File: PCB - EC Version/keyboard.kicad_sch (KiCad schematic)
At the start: 98 parts, among them J1 HRO_TYPE-C-31-M-12, J2 Conn_01x03, SW1 Alps SKRK, SW2 Alps SKRK, U1 TLV75533PDBV, U101 RP2040, U103 W25Q16, Y1 12MHz 3225 20pF

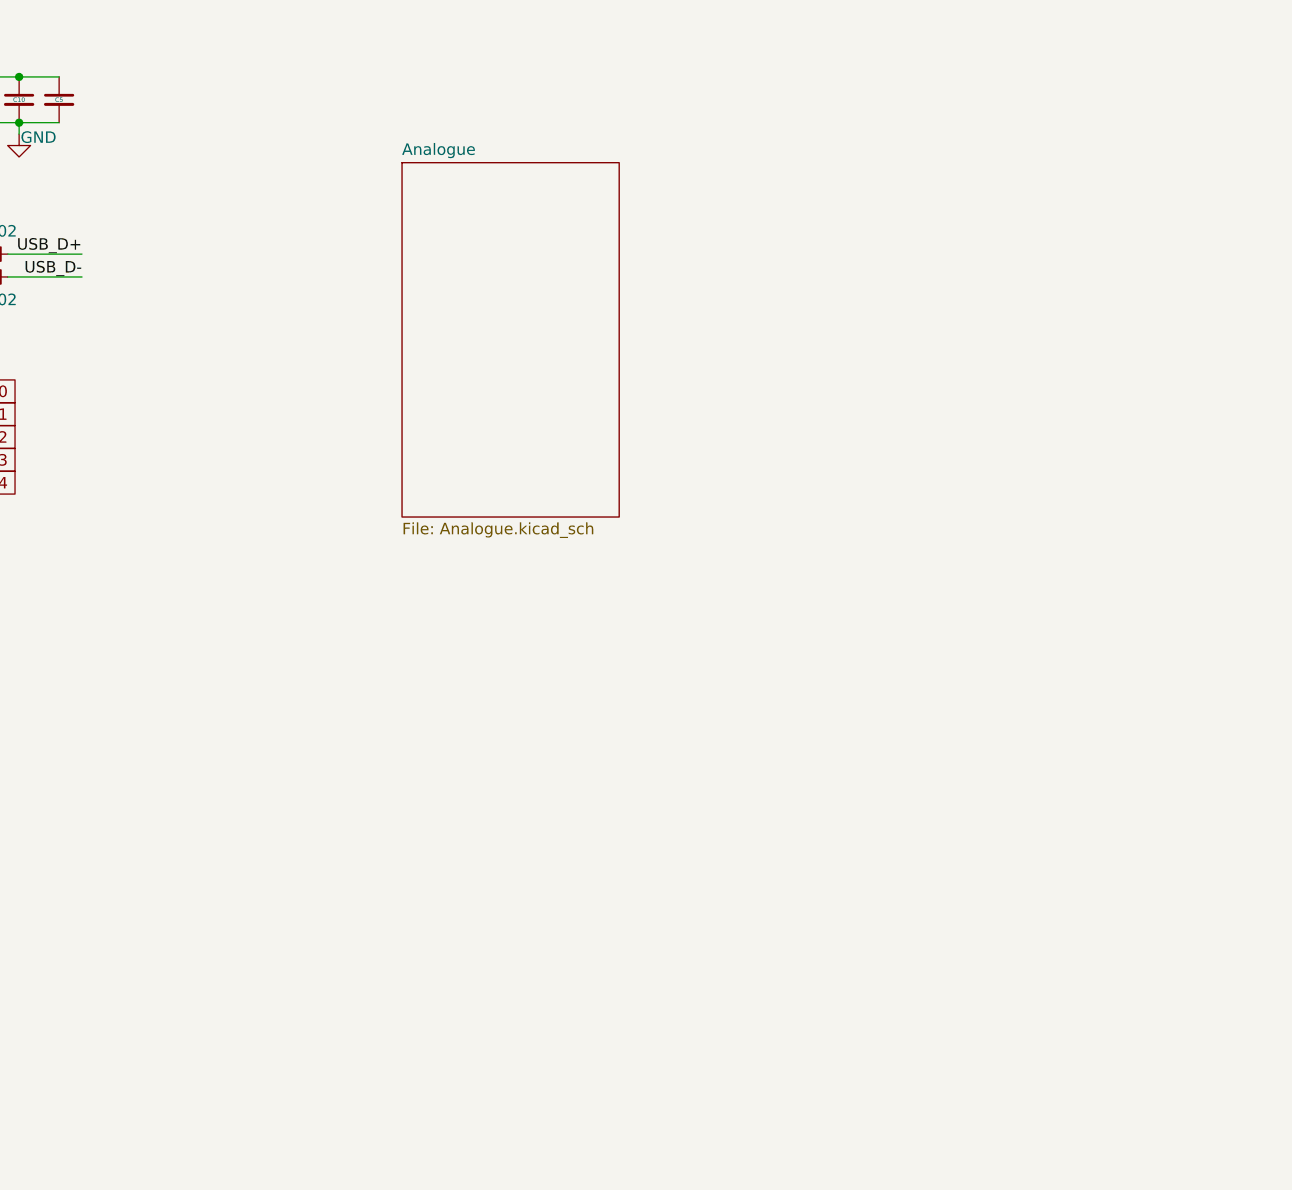
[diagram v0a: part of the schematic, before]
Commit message: couple extra bits
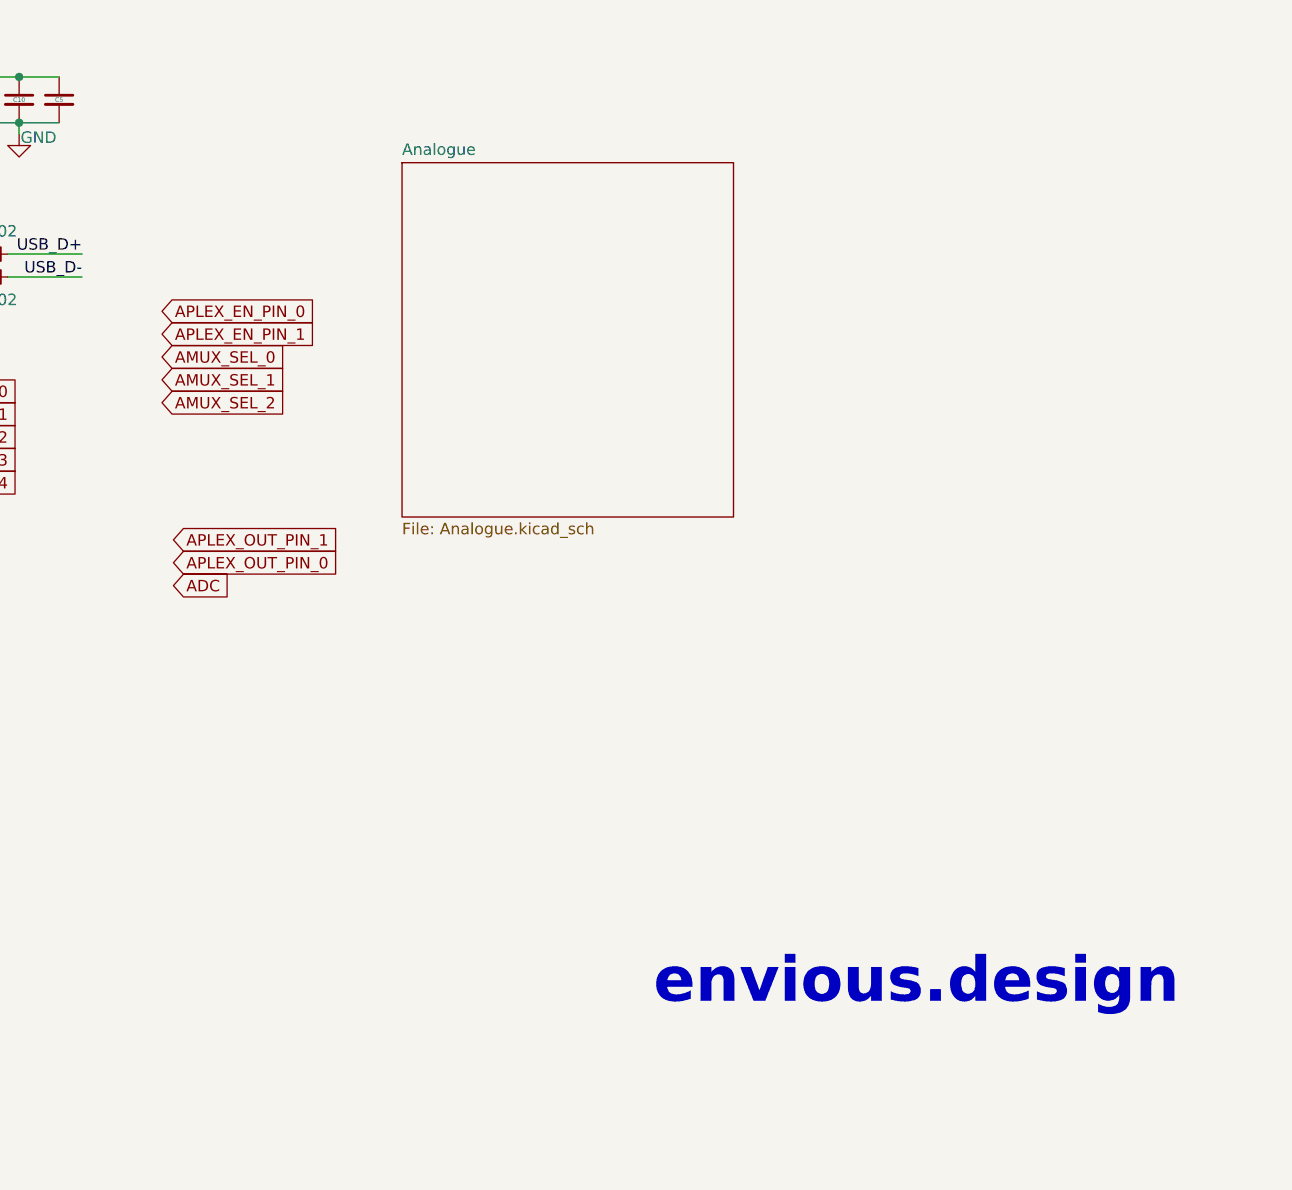
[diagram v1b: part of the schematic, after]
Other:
- note added: "envious.design"
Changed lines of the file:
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@@
     )
   )
+  (text "envious.design" (at 359.41 262.89 0)
+    (effects (font (face "Dissolve light") (size 5 5) (thickness 1) bold) (justify left bottom) (href "http://envious.design"))
+  )
   (label "USB_D+" (at 53.975 200.66 180) (fields_autoplaced)
     (effects (font (size 1.27 1.27)) (justify right bottom))
@@
     (effects (font (size 1.27 1.27)) (justify right bottom))
   )
+  (global_label "ADC" (shape input) (at 306.07 215.9 0) (fields_autoplaced)
+    (effects (font (size 1.27 1.27)) (justify left))
+    (property "Intersheetrefs" "${INTERSHEET_REFS}" (at 312.1117 215.8206 0)
+      (effects (font (size 1.27 1.27)) (justify left) hide)
+    )
+  )
   (global_label "col4" (shape input) (at 147.32 16.51 180)
     (effects (font (size 1.27 1.27)) (justify right))
@@
     )
   )
+  (global_label "APLEX_EN_PIN_1" (shape input) (at 304.8 187.96 0) (fields_autoplaced)
+    (effects (font (size 1.27 1.27)) (justify left))
+    (property "Intersheetrefs" "${INTERSHEET_REFS}" (at 322.7555 187.8806 0)
+      (effects (font (size 1.27 1.27)) (justify left) hide)
+    )
+  )
   (global_label "row3" (shape input) (at 22.86 111.76 180)
     (effects (font (size 1.27 1.27)) (justify right))
@@
     )
   )
+  (global_label "AMUX_SEL_1" (shape input) (at 304.8 193.04 0) (fields_autoplaced)
+    (effects (font (size 1.27 1.27)) (justify left))
+    (property "Intersheetrefs" "${INTERSHEET_REFS}" (at 318.8245 192.9606 0)
+      (effects (font (size 1.27 1.27)) (justify left) hide)
+    )
+  )
   (global_label "QSPI_SD1" (shape input) (at 218.44 196.85 180) (fields_autoplaced)
     (effects (font (size 1.27 1.27)) (justify right))
@@
     )
   )
+  (global_label "AMUX_SEL_2" (shape input) (at 304.8 195.58 0) (fields_autoplaced)
+    (effects (font (size 1.27 1.27)) (justify left))
+    (property "Intersheetrefs" "${INTERSHEET_REFS}" (at 318.8245 195.5006 0)
+      (effects (font (size 1.27 1.27)) (justify left) hide)
+    )
+  )
+  (global_label "APLEX_OUT_PIN_0" (shape input) (at 306.07 213.36 0) (fields_autoplaced)
+    (effects (font (size 1.27 1.27)) (justify left))
+    (property "Intersheetrefs" "${INTERSHEET_REFS}" (at 325.1745 213.2806 0)
+      (effects (font (size 1.27 1.27)) (justify left) hide)
+    )
+  )
+  (global_label "APLEX_EN_PIN_0" (shape input) (at 304.8 185.42 0) (fields_autoplaced)
+    (effects (font (size 1.27 1.27)) (justify left))
+    (property "Intersheetrefs" "${INTERSHEET_REFS}" (at 322.7555 185.3406 0)
+      (effects (font (size 1.27 1.27)) (justify left) hide)
+    )
+  )
   (global_label "col13" (shape input) (at 375.92 16.51 180)
     (effects (font (size 1.27 1.27)) (justify right))
@@
     )
   )
+  (global_label "APLEX_OUT_PIN_1" (shape input) (at 306.07 210.82 0) (fields_autoplaced)
+    (effects (font (size 1.27 1.27)) (justify left))
+    (property "Intersheetrefs" "${INTERSHEET_REFS}" (at 325.1745 210.7406 0)
+      (effects (font (size 1.27 1.27)) (justify left) hide)
+    )
+  )
   (global_label "col12" (shape input) (at 350.52 16.51 180)
     (effects (font (size 1.27 1.27)) (justify right))
@@
     )
   )
+  (global_label "AMUX_SEL_0" (shape input) (at 304.8 190.5 0) (fields_autoplaced)
+    (effects (font (size 1.27 1.27)) (justify left))
+    (property "Intersheetrefs" "${INTERSHEET_REFS}" (at 318.8245 190.4206 0)
+      (effects (font (size 1.27 1.27)) (justify left) hide)
+    )
+  )
   (global_label "QSPI_SD1" (shape input) (at 171.45 194.31 180) (fields_autoplaced)
     (effects (font (size 1.27 1.27)) (justify right))
@@
     )
   )
-  (sheet (at 331.47 168.91) (size 24.13 39.37) (fields_autoplaced)
+  (sheet (at 331.47 168.91) (size 36.83 39.37) (fields_autoplaced)
     (stroke (width 0.1524) (type solid))
     (fill (color 0 0 0 0.0000))
